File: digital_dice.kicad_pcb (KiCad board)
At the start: 2 copper layers, 23 parts, among them J1 Barrel_Jack, SW1 SW_SPST, SW2 SW_SPST, U1 NE555D, U2 74LS90, U3 74LS47, U4 SC39-11EWA, U5 LM7805_TO220, U6 74LS11

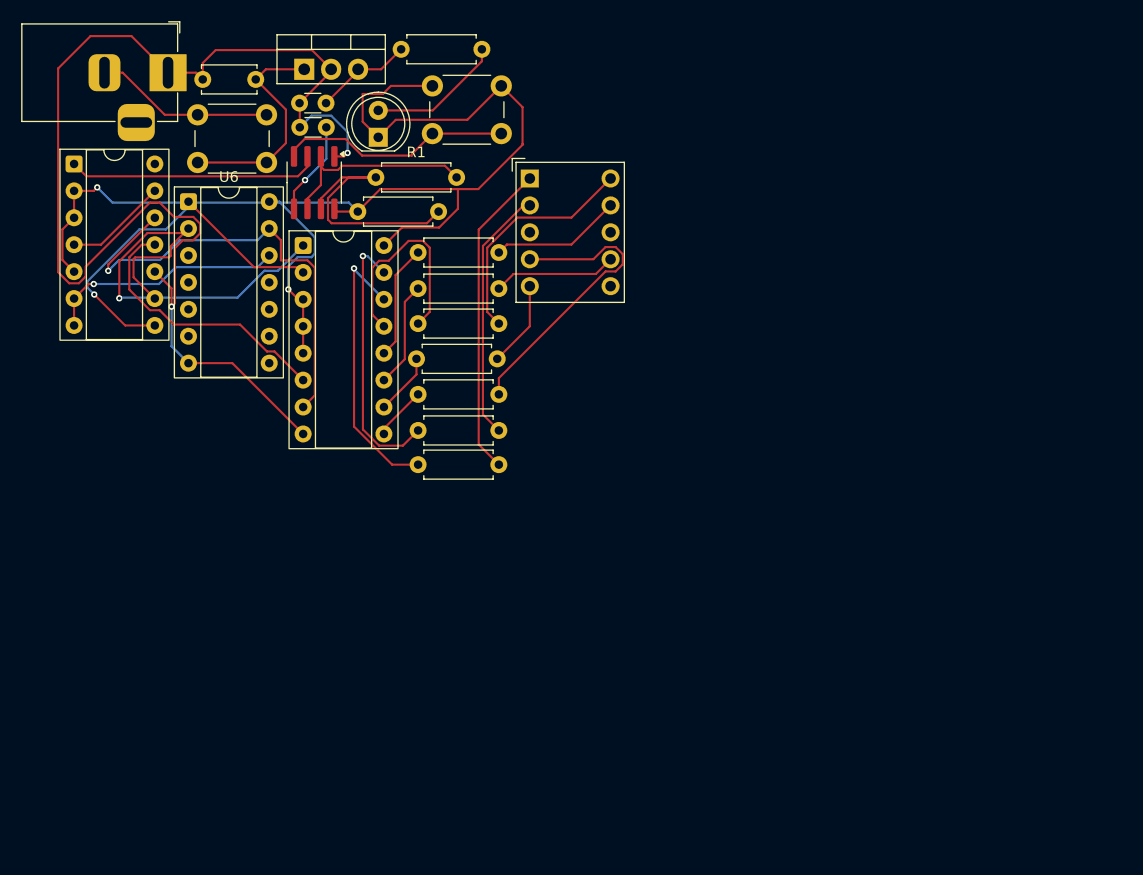
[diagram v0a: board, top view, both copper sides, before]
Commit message: Final Touches:
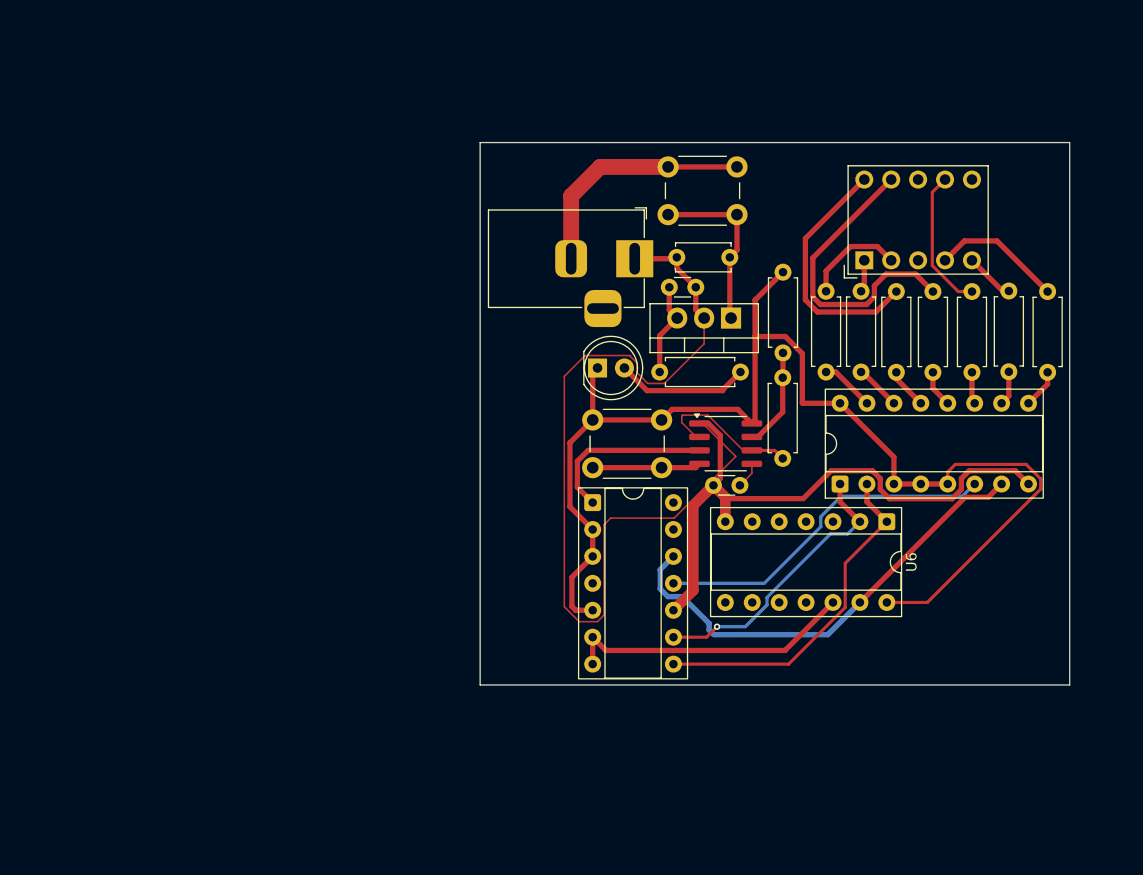
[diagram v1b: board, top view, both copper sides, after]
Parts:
- moved U6 72.5 mm to (154.1, 92.4), turned to -90 degrees
- moved R7 59.4 mm to (169.3, 78.3), turned to 90 degrees
- moved U2 58.4 mm to (126.4, 90.6)
- moved R6 55.9 mm to (165.6, 78.3), turned to 90 degrees
- moved U3 55.4 mm to (149.7, 88.8), turned to 90 degrees
- moved R4 52.9 mm to (162.1, 78.3), turned to 90 degrees
- moved C4 51.6 mm to (137.7, 89.0)
- moved R3 49.9 mm to (158.5, 78.3), turned to 90 degrees
- moved C5 47.8 mm to (134.3, 67.5)
- moved J1 47.4 mm to (130.3, 67.6)
- moved U5 46.6 mm to (139.4, 73.2), turned to 180 degrees
- moved U1 46.0 mm to (138.9, 85.0), turned to 0 degrees
- moved R5 45.4 mm to (155.0, 78.3), turned to 90 degrees
- moved SW2 44.7 mm to (133.5, 58.9)
- moved R1 42.8 mm to (144.3, 78.8), turned to -90 degrees
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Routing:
- net GND: track 118.5 -> 147.6 mm, vias 2 -> 0
- net Net-(U4-G): track 29.8 -> 3.05 mm
- net Net-(U3-g): track 26.5 -> 4.32 mm, vias 1 -> 0
- net Net-(U3-f): track 25.4 -> 5.08 mm, vias 1 -> 0
- net Net-(U3-a): track 20.4 -> 3.88 mm
- net Net-(U1-DIS): track 25.9 -> 9.47 mm
- net Net-(U4-B): track 12.4 -> 28.2 mm
- net Net-(U4-E): track 28.2 -> 12.4 mm
- net Net-(U2-Q1): track 42.2 -> 26.9 mm
- net Net-(U4-F): track 24.0 -> 9.56 mm
- net Net-(SW1-B): track 22.2 -> 10.2 mm
- net (no net): track 9.72 -> 0.00 mm
- net Net-(U1-Q): track 23.9 -> 16.4 mm
- net Net-(U3-b): track 10.8 -> 3.50 mm
- net Net-(U2-Q3): track 25.9 -> 32.9 mm
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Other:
- board outline added: 55.6 x 51.2 mm

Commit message: Update PCB layout
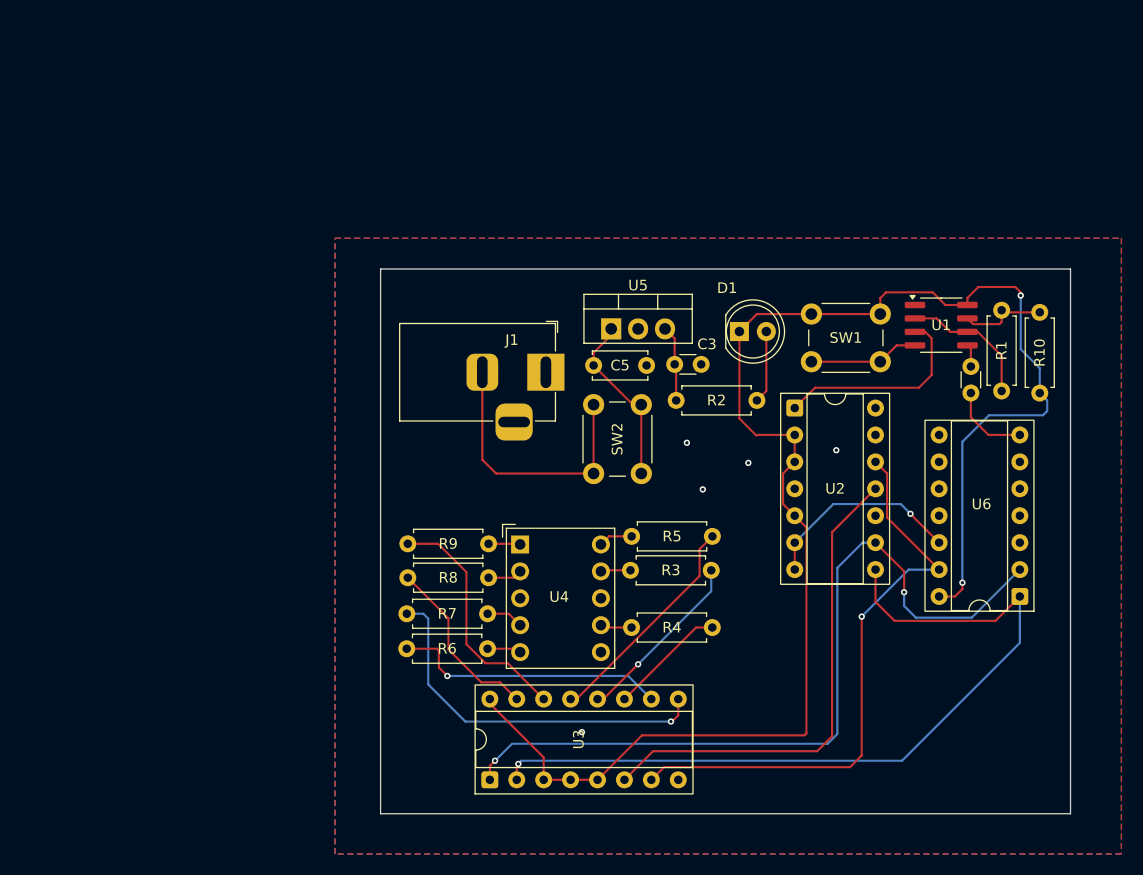
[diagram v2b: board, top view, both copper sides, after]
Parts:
- moved R7 64.6 mm to (108.8, 101.1), turned to 0 degrees
- moved R6 62.5 mm to (108.8, 104.4), turned to 0 degrees
- moved R9 45.7 mm to (108.9, 94.5), turned to 0 degrees
- moved R8 44.0 mm to (108.9, 97.7), turned to 0 degrees
- moved U3 43.3 mm to (116.7, 116.8)
- moved U4 42.1 mm to (119.5, 94.5), turned to 0 degrees
- moved R4 34.4 mm to (137.6, 102.4), turned to 180 degrees
- moved SW2 29.8 mm to (126.4, 87.9), turned to 90 degrees
- moved R3 28.0 mm to (137.5, 97.0), turned to 180 degrees
- moved R10 26.8 mm to (168.5, 80.3), turned to 90 degrees
- moved C4 25.8 mm to (162.0, 80.3), turned to 90 degrees
- moved R5 23.3 mm to (137.7, 93.8), turned to 180 degrees
- moved U1 23.2 mm to (159.2, 73.9)
- moved SW1 22.9 mm to (147.0, 72.8)
- moved R1 21.6 mm to (164.9, 72.5)
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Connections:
- net Net-(D1-K) renamed /+5V
- net Net-(U1-DIS) renamed /DIS
- net Net-(U1-Q) renamed /Q
- net Net-(U1-THR) renamed /TR/THR
- net Net-(U2-Q0) renamed /Q0
- net Net-(U2-Q1) renamed /Q1
- net Net-(U2-Q2) renamed /Q2
- net Net-(U2-Q3) renamed /Q3
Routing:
- net GND: track 147.6 -> 7.61 mm, vias 0 -> 5
- net /Q1: track 26.9 -> 76.0 mm, vias 1 -> 2
- net /Q2: track 32.5 -> 76.4 mm, vias 0 -> 1
- net Net-(U3-e): track 3.67 -> 35.2 mm, vias 0 -> 1
- net /+5V: track 117.7 -> 149.2 mm, vias 0 -> 2
- net Net-(U4-B): track 28.2 -> 2.83 mm
- net Net-(U3-d): track 3.26 -> 26.0 mm, vias 0 -> 1
- net Net-(U4-A): track 23.5 -> 3.21 mm
- net Net-(U3-g): track 4.32 -> 22.9 mm
- net Net-(U3-a): track 3.88 -> 21.2 mm
- net /Q3: track 32.9 -> 46.3 mm
- net Net-(U3-b): track 3.50 -> 16.9 mm, vias 0 -> 1
- net /Q0: track 43.8 -> 55.7 mm, vias 0 -> 1
- net Net-(U3-f): track 5.08 -> 16.7 mm
- net Net-(U4-C): track 13.4 -> 2.98 mm
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- added copper zone on B.Cu, net GND
- added copper zone on F.Cu, net GND
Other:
- board size 55.6 x 51.2 mm -> 65.1 x 51.4 mm
